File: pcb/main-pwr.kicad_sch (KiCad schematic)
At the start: 6 parts

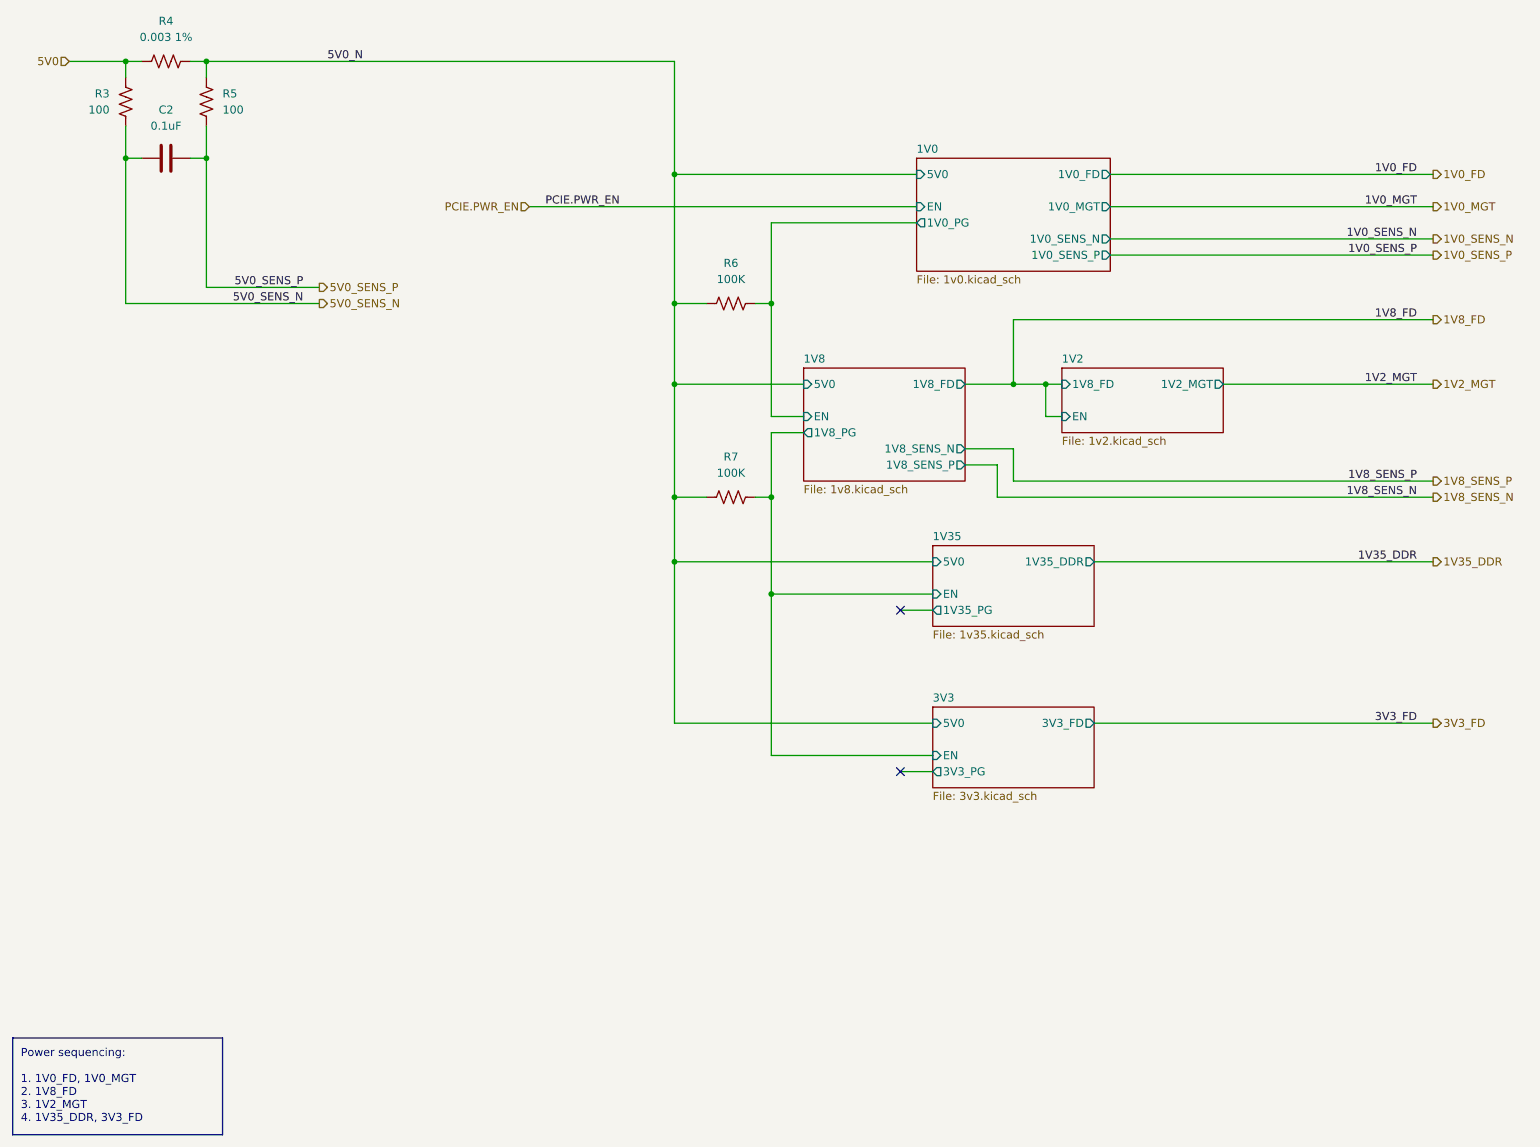
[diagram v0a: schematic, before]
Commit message: jtag, dcplng
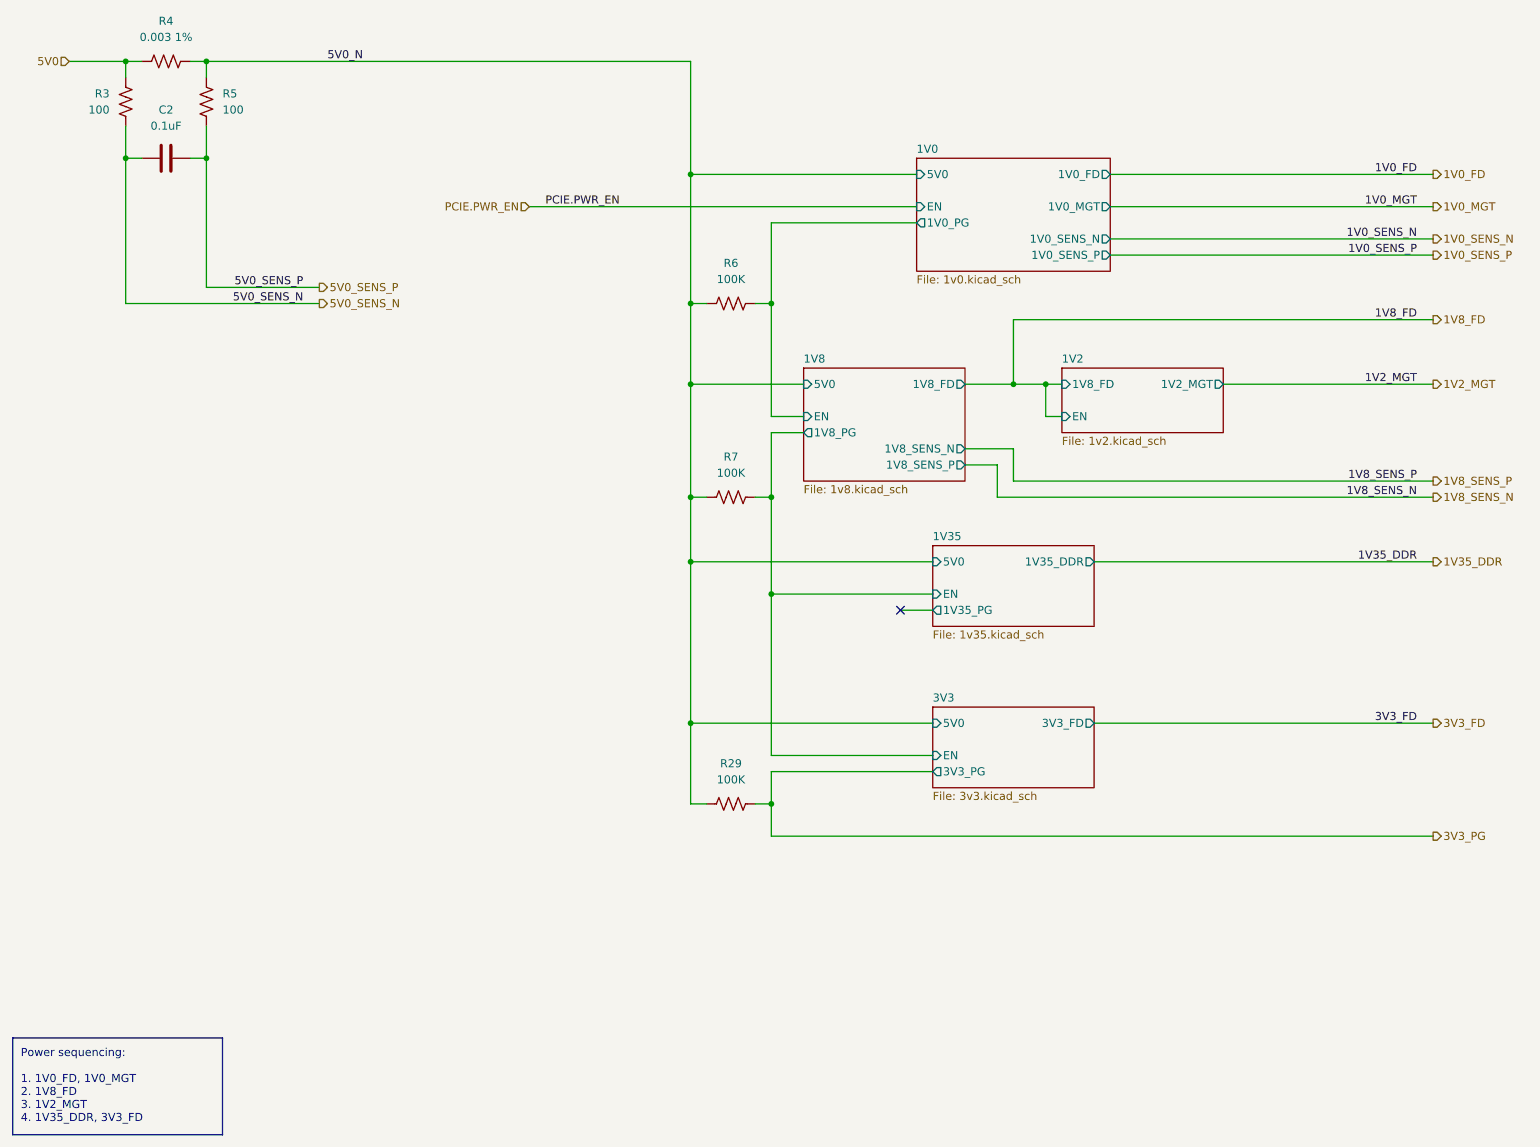
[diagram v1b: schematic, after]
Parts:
- added R29: 100K, library:R_0402_1005Metric, symbol library:R_US
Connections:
- net 5V0_N: now also R29.1
- new net 3V3_PG: R29.2
- no-connect marks 2 -> 1
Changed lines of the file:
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@@
 	)
 	(junction
-		(at 119.38 104.14)
+		(at 121.92 104.14)
 		(diameter 0)
 		(color 255 0 0 1)
@@
 	)
 	(junction
-		(at 119.38 93.98)
+		(at 134.62 142.24)
+		(diameter 0)
+		(color 0 0 0 0)
+	)
+	(junction
+		(at 121.92 93.98)
 		(diameter 0)
 		(color 255 0 0 1)
@@
 	)
 	(junction
-		(at 119.38 63.5)
+		(at 121.92 63.5)
 		(diameter 0)
 		(color 255 0 0 1)
 	)
 	(junction
-		(at 119.38 76.2)
+		(at 121.92 76.2)
 		(diameter 0)
 		(color 255 0 0 1)
@@
 	)
 	(junction
-		(at 119.38 43.18)
+		(at 121.92 43.18)
 		(diameter 0)
 		(color 255 0 0 1)
@@
 	)
 	(junction
+		(at 121.92 129.54)
+		(diameter 0)
+		(color 255 0 0 1)
+	)
+	(junction
 		(at 134.62 109.22)
 		(diameter 0)
@@
 	)
 	(no_connect
-		(at 154.94 137.16)
-	)
-	(no_connect
 		(at 154.94 111.76)
 	)
@@
 	(wire
 		(pts
-			(xy 119.38 93.98) (xy 124.46 93.98)
+			(xy 121.92 93.98) (xy 124.46 93.98)
 		)
 		(stroke
@@
 	(wire
 		(pts
+			(xy 134.62 142.24) (xy 134.62 147.32)
+		)
+		(stroke
+			(width 0)
+			(type default)
+		)
+	)
+	(wire
+		(pts
 			(xy 187.96 48.26) (xy 238.76 48.26)
 		)
@@
 	(wire
 		(pts
-			(xy 154.94 137.16) (xy 160.02 137.16)
+			(xy 121.92 129.54) (xy 121.92 142.24)
+		)
+		(stroke
+			(width 0.3556)
+			(type default)
+			(color 255 0 0 1)
+		)
+	)
+	(wire
+		(pts
+			(xy 134.62 137.16) (xy 160.02 137.16)
 		)
 		(stroke
@@
 	(wire
 		(pts
+			(xy 132.08 142.24) (xy 134.62 142.24)
+		)
+		(stroke
+			(width 0)
+			(type default)
+		)
+	)
+	(wire
+		(pts
 			(xy 172.72 76.2) (xy 172.72 66.04)
 		)
@@
 	(wire
 		(pts
-			(xy 119.38 93.98) (xy 119.38 104.14)
+			(xy 121.92 93.98) (xy 121.92 104.14)
 		)
 		(stroke
@@
 	(wire
 		(pts
+			(xy 121.92 142.24) (xy 124.46 142.24)
+		)
+		(stroke
+			(width 0.3556)
+			(type default)
+			(color 255 0 0 1)
+		)
+	)
+	(wire
+		(pts
 			(xy 177.8 76.2) (xy 180.34 76.2)
 		)
@@
 	(wire
 		(pts
-			(xy 119.38 76.2) (xy 119.38 93.98)
+			(xy 134.62 147.32) (xy 238.76 147.32)
+		)
+		(stroke
+			(width 0)
+			(type default)
+		)
+	)
+	(wire
+		(pts
+			(xy 121.92 76.2) (xy 121.92 93.98)
 		)
 		(stroke
@@
 	(wire
 		(pts
-			(xy 45.72 25.4) (xy 119.38 25.4)
+			(xy 45.72 25.4) (xy 121.92 25.4)
 		)
 		(stroke
@@
 	(wire
 		(pts
-			(xy 119.38 25.4) (xy 119.38 43.18)
+			(xy 121.92 25.4) (xy 121.92 43.18)
 		)
 		(stroke
@@
 	(wire
 		(pts
-			(xy 119.38 43.18) (xy 119.38 63.5)
+			(xy 121.92 43.18) (xy 121.92 63.5)
 		)
 		(stroke
@@
 	(wire
 		(pts
-			(xy 119.38 63.5) (xy 124.46 63.5)
+			(xy 121.92 63.5) (xy 124.46 63.5)
 		)
 		(stroke
@@
 	(wire
 		(pts
-			(xy 119.38 76.2) (xy 139.7 76.2)
+			(xy 121.92 76.2) (xy 139.7 76.2)
 		)
 		(stroke
@@
 	(wire
 		(pts
+			(xy 134.62 137.16) (xy 134.62 142.24)
+		)
+		(stroke
+			(width 0)
+			(type default)
+		)
+	)
+	(wire
+		(pts
 			(xy 154.94 111.76) (xy 160.02 111.76)
 		)
@@
 	(wire
 		(pts
-			(xy 119.38 43.18) (xy 157.48 43.18)
+			(xy 121.92 43.18) (xy 157.48 43.18)
 		)
 		(stroke
@@
 	(wire
 		(pts
-			(xy 119.38 63.5) (xy 119.38 76.2)
+			(xy 121.92 63.5) (xy 121.92 76.2)
 		)
 		(stroke
@@
 	(wire
 		(pts
-			(xy 119.38 104.14) (xy 119.38 129.54)
+			(xy 121.92 104.14) (xy 121.92 129.54)
 		)
 		(stroke
@@
 	(wire
 		(pts
-			(xy 119.38 104.14) (xy 160.02 104.14)
+			(xy 121.92 104.14) (xy 160.02 104.14)
 		)
 		(stroke
@@
 	(wire
 		(pts
-			(xy 119.38 129.54) (xy 160.02 129.54)
+			(xy 121.92 129.54) (xy 160.02 129.54)
 		)
 		(stroke
@@
 		(shape output)
 		(at 238.76 76.2 0)
+		(effects
+			(font
+				(size 1.27 1.27)
+			)
+			(justify left)
+		)
+	)
+	(hierarchical_label "3V3_PG"
+		(shape output)
+		(at 238.76 147.32 0)
 		(effects
 			(font
@@
 	(symbol
 		(lib_id "library:R_US")
+		(at 128.27 142.24 90)
+		(unit 1)
+		(exclude_from_sim no)
+		(in_bom yes)
+		(on_board yes)
+		(dnp no)
+		(fields_autoplaced yes)
+		(property "Reference" "R29"
+			(at 128.27 135.89 90)
+			(effects
+				(font
+					(size 1.27 1.27)
+				)
+			)
+		)
+		(property "Value" "100K"
+			(at 128.27 138.43 90)
+			(effects
+				(font
+					(size 1.27 1.27)
+				)
+			)
+		)
+		(property "Footprint" "library:R_0402_1005Metric"
+			(at 128.524 141.224 90)
+			(effects
+				(font
+					(size 1.27 1.27)
+				)
+				(hide yes)
+			)
+		)
+		(property "Datasheet" "~"
+			(at 128.27 142.24 0)
+			(effects
+				(font
+					(size 1.27 1.27)
+				)
+				(hide yes)
+			)
+		)
+		(property "Description" "RES 100K OHM 1% 1/16W 0402"
+			(at 128.27 142.24 0)
+			(effects
+				(font
+					(size 1.27 1.27)
+				)
+				(hide yes)
+			)
+		)
+		(property "Manufacturer" "YAGEO"
+			(at 128.27 142.24 0)
+			(effects
+				(font
+					(size 1.27 1.27)
+				)
+				(hide yes)
+			)
+		)
+		(property "Manufacturer Product Number" "RC0402FR-07100KL"
+			(at 128.27 142.24 90)
+			(effects
+				(font
+					(size 1.27 1.27)
+				)
+				(hide yes)
+			)
+		)
+		(pin "2"
+		)
+		(pin "1"
+		)
+		(instances
+			(project "RPi-HwAB-1"
+				(path "/e63e39d7-6ac0-4ffd-8aa3-1841a4541b55/f9ebb56c-78c7-42ac-bc19-ccbf788f5318"
+					(reference "R29")
+					(unit 1)
+				)
+			)
+		)
+	)
+	(symbol
+		(lib_id "library:R_US")
 		(at 39.37 25.4 90)
 		(unit 1)
@@
 		)
 		(fill
-			(color 0 0 0 0.0000)
+			(color 132 0 0 0.0588)
 		)
 		(property "Sheetname" "1V2"
@@
 		)
 		(fill
-			(color 0 0 0 0.0000)
+			(color 132 0 0 0.0588)
 		)
 		(property "Sheetname" "1V8"
@@
 		)
 		(fill
-			(color 0 0 0 0.0000)
+			(color 132 0 0 0.0600)
 		)
 		(property "Sheetname" "1V0"
@@
 		)
 		(fill
-			(color 0 0 0 0.0000)
+			(color 132 0 0 0.0588)
 		)
 		(property "Sheetname" "3V3"
@@
 		)
 		(fill
-			(color 0 0 0 0.0000)
+			(color 132 0 0 0.0588)
 		)
 		(property "Sheetname" "1V35"
